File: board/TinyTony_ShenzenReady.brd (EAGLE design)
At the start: 39 x 35.5 mm, 7 parts, among them U1 ATTINY85

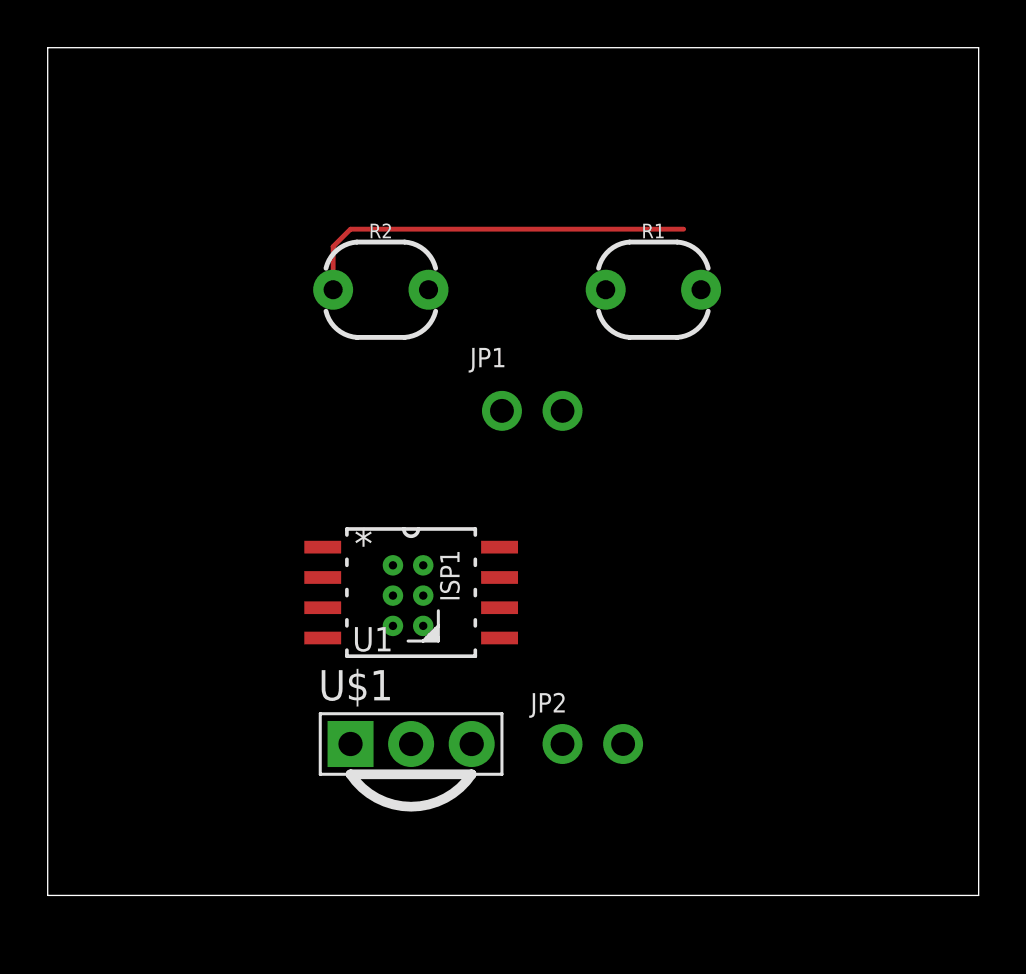
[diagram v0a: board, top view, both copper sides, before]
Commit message: yet another layout
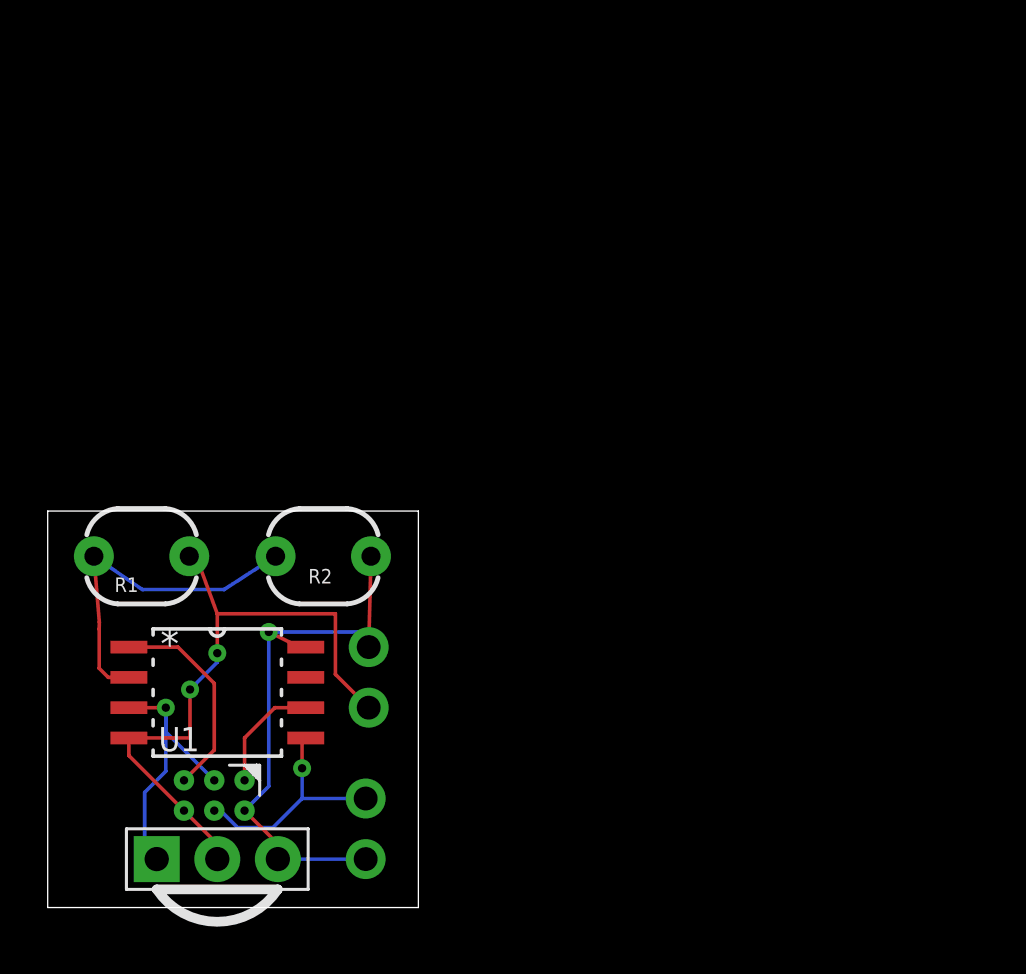
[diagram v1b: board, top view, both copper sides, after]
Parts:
- moved R1 24.2 mm to (3.94, 14.2), turned to 180 degrees
- moved ISP1 13.5 mm to (5.71, 3.56), turned to 270 degrees
- moved JP1 13.1 mm to (13.5, 9.14), turned to 270 degrees
- moved R2 11.4 mm to (11.6, 14.2)
- moved JP2 10.2 mm to (13.3, 2.79), turned to 270 degrees
- moved U$1 9.45 mm to (7.11, 1.52)
- moved U1 9.14 mm to (7.11, 8.51)
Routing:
- net GND: track 0.00 -> 27.0 mm, vias 0 -> 2
- net VCC: track 0.00 -> 24.5 mm, vias 0 -> 1
- net 3: track 0.00 -> 12.4 mm, vias 0 -> 1
- net 5: track 0.00 -> 9.75 mm, vias 0 -> 1
- net 1: track 0.00 -> 8.80 mm
- net 6: track 0.00 -> 4.87 mm
- net 2: track 16.8 -> 14.6 mm
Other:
- board size 39 x 35.5 mm -> 15.5 x 16.6 mm
